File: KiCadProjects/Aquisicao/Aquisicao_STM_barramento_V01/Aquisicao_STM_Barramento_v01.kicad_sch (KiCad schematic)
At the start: 13 parts, among them J1 alimentacao analogica, J2 sinais analogicos, J3 comunicacao / sinais digitais, J4 Conn_01x02, U1 BluePill_STM32F103C, U2 LM2596S-5, U3 LM1117T-3.3

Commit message: modificar
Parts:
- added J5: Conn_01x02, symbol Connector_Generic:Conn_01x02
- added U4, U5, U6: BluePill_STM32F103C, BluePill_breakouts:BluePill_STM32F103C, symbol bluepill_breakouts:BluePill_STM32F103C
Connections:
- net 3.3V_step: now also U4.40 (VCC3V3), U5.40 (VCC3V3), U6.40 (VCC3V3)
- net Ampl1: now also U1.6 (PA1), U4.6 (PA1), U5.6 (PA1), U6.6 (PA1); no longer U1.13 (PB0)
- net Ampl2: now also U1.9 (PA4), U4.9 (PA4), U5.9 (PA4), U6.9 (PA4); no longer U1.14 (PB1)
- net Earth: now also U4.20 (GND), U5.20 (GND), U6.20 (GND)
- net SCL1: now also U4.36 (PB8), U5.36 (PB8), U6.36 (PB8)
- net SDA1: now also U4.37 (PB9), U5.37 (PB9), U6.37 (PB9)
- net SINCD: now also U1.3 (PC14), U4.3 (PC14), U5.3 (PC14), U6.3 (PC14)
- net SINC_A: now also U1.10 (PA5_SCK1), U4.10 (PA5_SCK1), U5.10 (PA5_SCK1), U6.10 (PA5_SCK1)
- net SINC_B: now also U1.11 (PA6_MISO1), U4.11 (PA6_MISO1), U5.11 (PA6_MISO1), U6.11 (PA6_MISO1)
- net SINC_C: now also U1.12 (PA7_MOSI1), U4.12 (PA7_MOSI1), U5.12 (PA7_MOSI1), U6.12 (PA7_MOSI1)
- net sign_E1: now also U4.5 (PA0)
- new net sign_E2: J5.1 (Pin_1), U5.5 (PA0)
- new net sign_E3: J5.2 (Pin_2), U6.5 (PA0)
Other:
- moved on the sheet: J4, U1

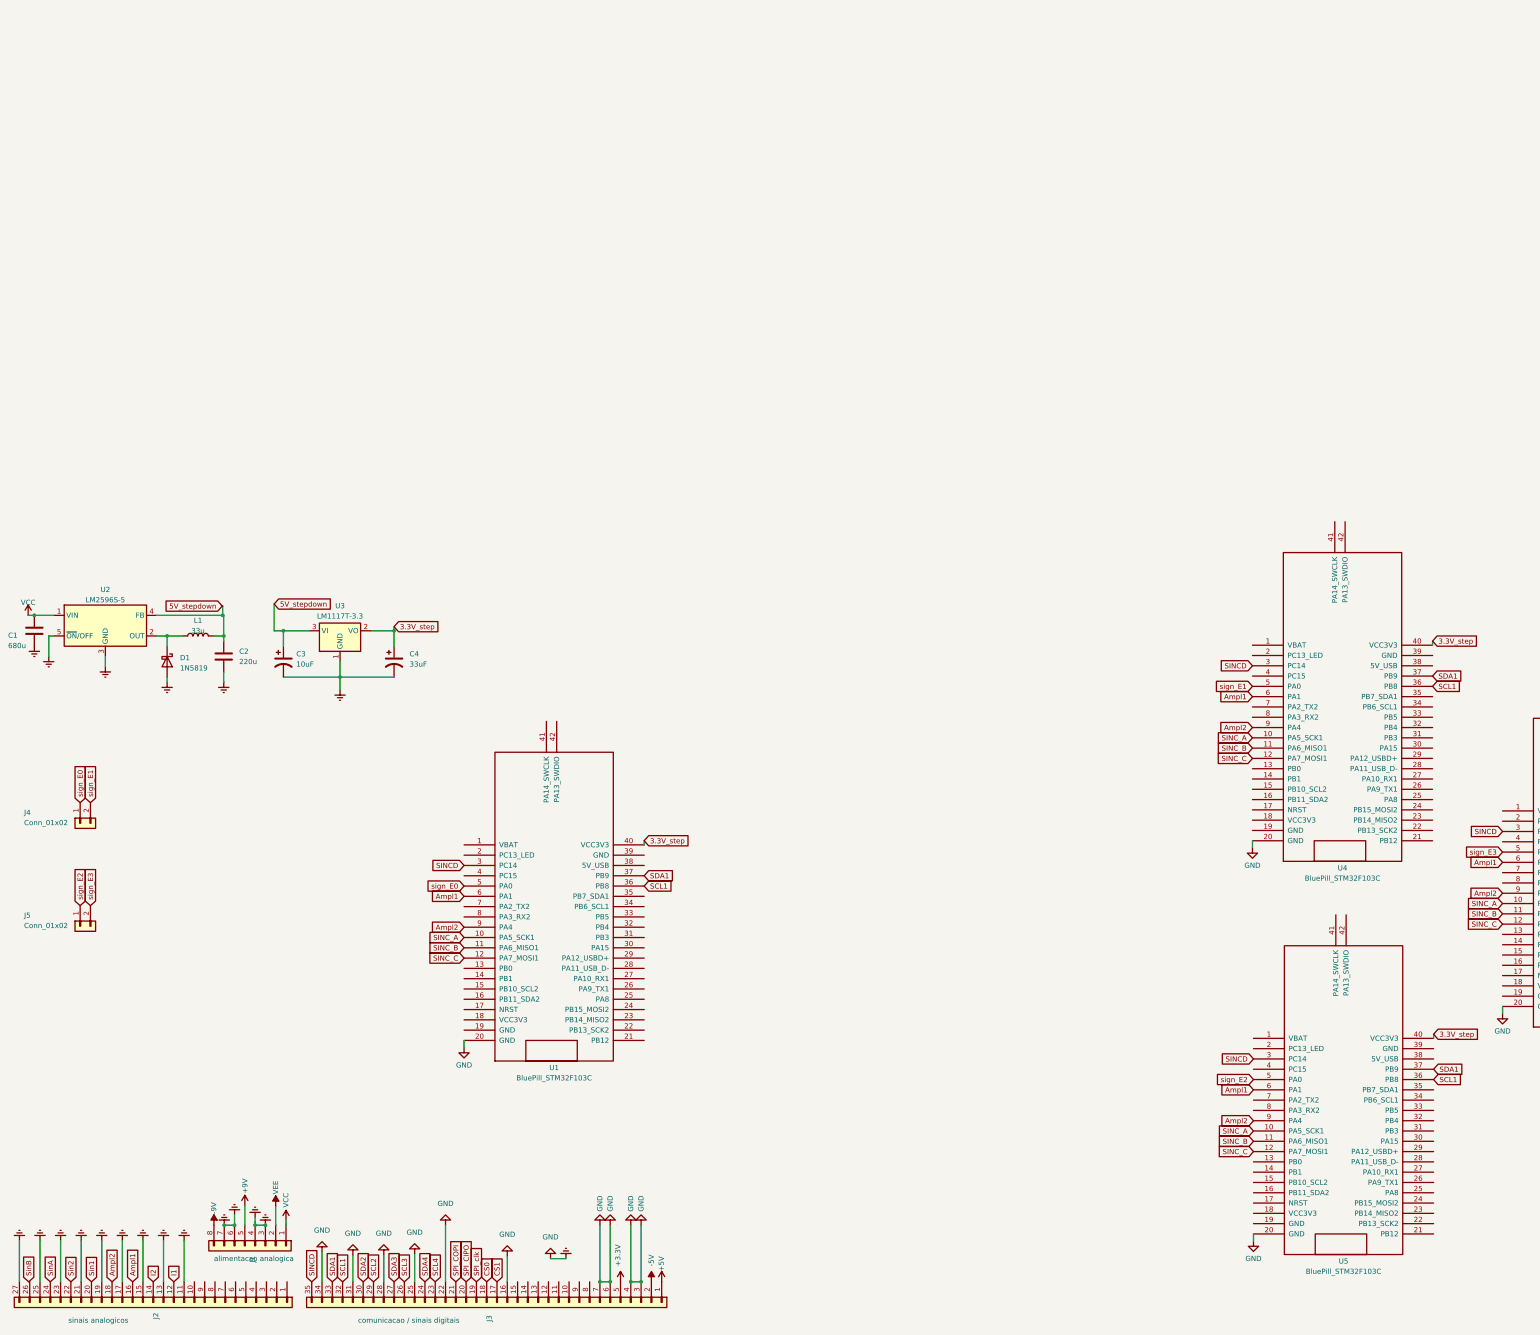
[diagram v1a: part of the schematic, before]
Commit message: tmp
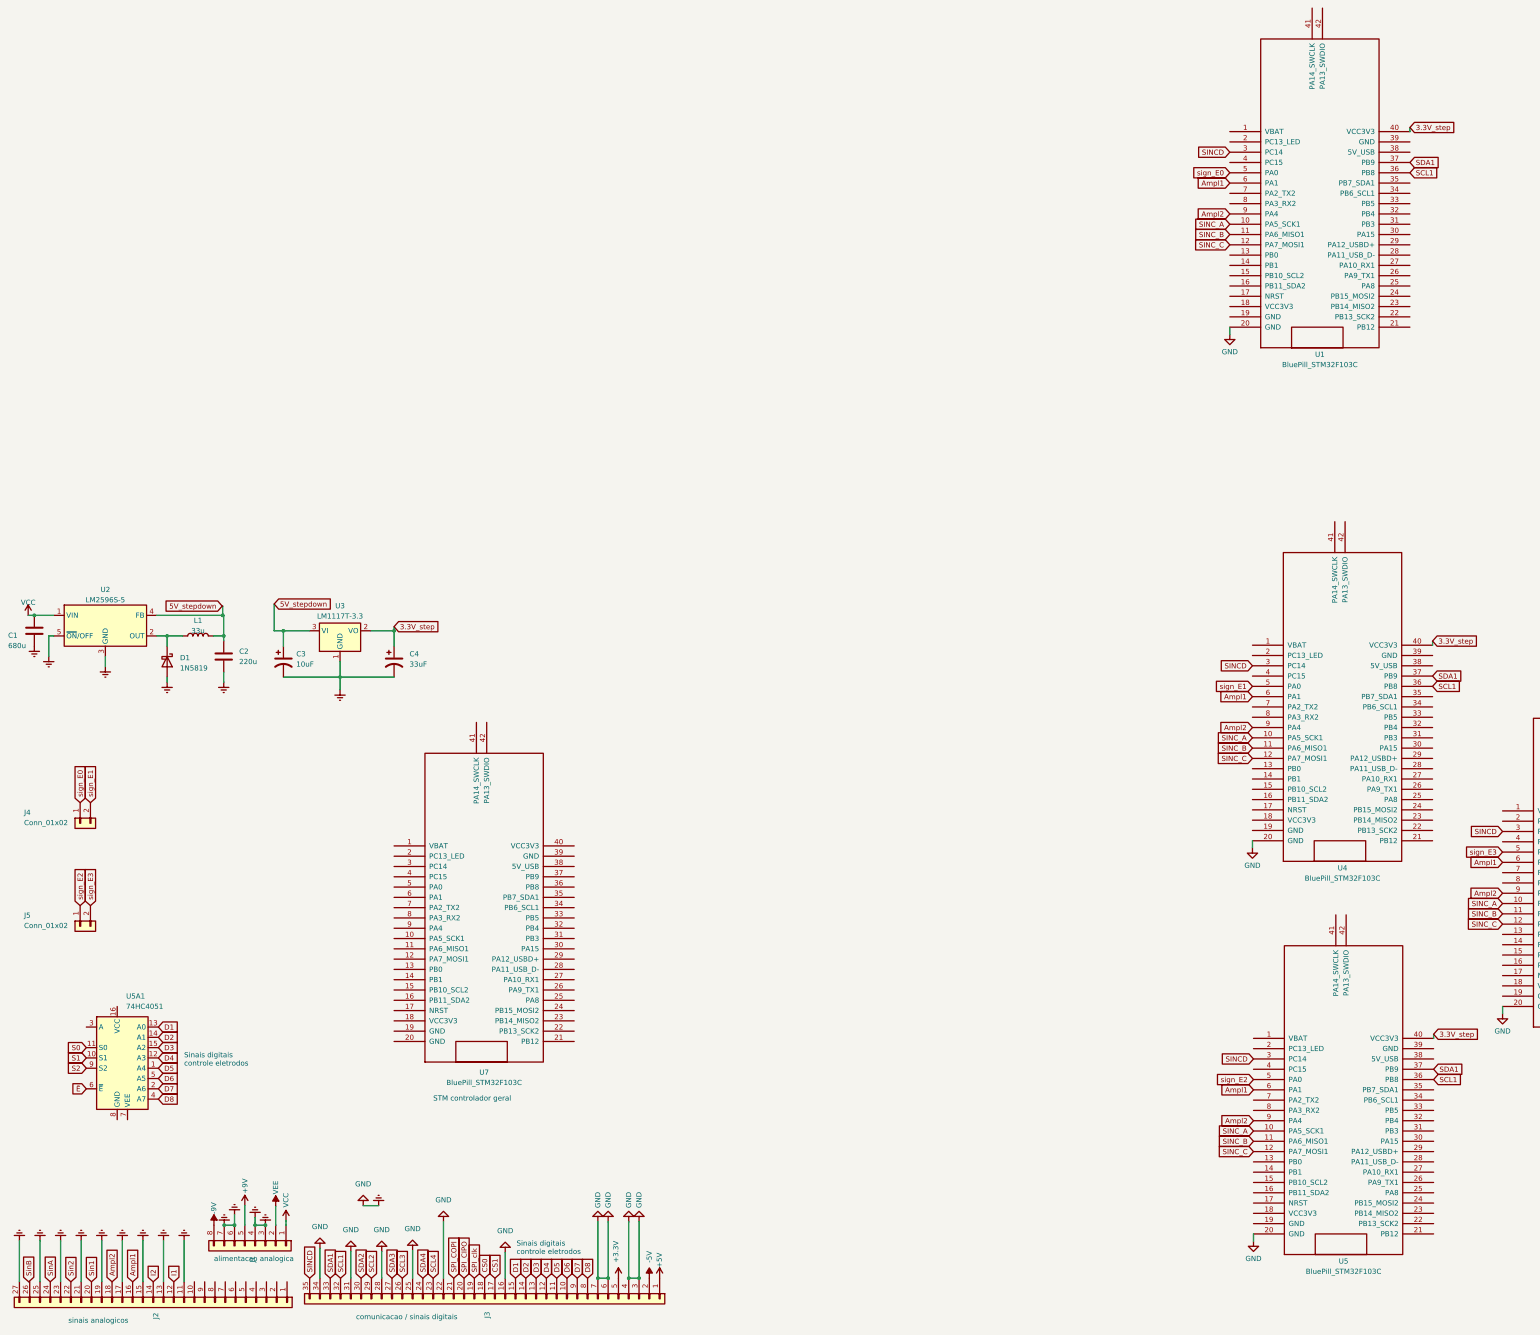
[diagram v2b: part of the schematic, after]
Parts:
- added U5A1: 74HC4051, 74HC4051N:N16, symbol 74xx:74HC4051
- added U7: BluePill_STM32F103C, BluePill_breakouts:BluePill_STM32F103C, symbol bluepill_breakouts:BluePill_STM32F103C
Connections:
- net D6: now reaches J3.10 (Pin_10)
- net D6: now also U5A1.5 (A5)
- net D5: now reaches J3.11 (Pin_11)
- net D5: now also U5A1.1 (A4)
- net D4: now reaches J3.12 (Pin_12)
- net D4: now also U5A1.12 (A3)
- net D3: now reaches J3.13 (Pin_13)
- net D3: now also U5A1.15 (A2)
- net D2: now reaches J3.14 (Pin_14)
- net D2: now also U5A1.14 (A1)
- net D1: now reaches J3.15 (Pin_15)
- net D1: now also U5A1.13 (A0)
- net D8: now reaches J3.8 (Pin_8)
- net D8: now also U5A1.4 (A7)
- net D7: now reaches J3.9 (Pin_9)
- net D7: now also U5A1.2 (A6)
- new net S0: U5A1.11 (S0)
- new net S1: U5A1.10 (S1)
- new net S2: U5A1.9 (S2)
- new net Ẽ: U5A1.6 (~{E})
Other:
- note added: "STM controlador geral"
- note added: "Sinais digitais controle eletrodos"
- moved on the sheet: J3, U1

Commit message: tmp
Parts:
- removed U5A1: 74HC4051, 74HC4051N:N16, symbol 74xx:74HC4051
- removed U7: BluePill_STM32F103C, BluePill_breakouts:BluePill_STM32F103C, symbol bluepill_breakouts:BluePill_STM32F103C
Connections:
- net D1 is gone; now on net SINC_A: J3.15 (Pin_15)
- net D2 is gone; now on net SINC_B: J3.14 (Pin_14)
- net D3 is gone; now on net SINC_C: J3.13 (Pin_13)
- net SCL1: now also U1.34 (PB6_SCL1), U4.34 (PB6_SCL1), U5.34 (PB6_SCL1), U6.34 (PB6_SCL1); no longer U1.36 (PB8), U4.36 (PB8), U5.36 (PB8), U6.36 (PB8)
- net SDA1: now also U1.35 (PB7_SDA1), U4.35 (PB7_SDA1), U5.35 (PB7_SDA1), U6.35 (PB7_SDA1); no longer U1.37 (PB9), U4.37 (PB9), U5.37 (PB9), U6.37 (PB9)
- net D4: no longer names the net of J3.12 (Pin_12)
- net D5: no longer names the net of J3.11 (Pin_11)
- net D6: no longer names the net of J3.10 (Pin_10)
- net D7: no longer names the net of J3.9 (Pin_9)
- net D8: no longer names the net of J3.8 (Pin_8)
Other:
- note removed: "STM controlador geral"
- note removed: "Sinais digitais controle eletrodos"
- moved on the sheet: C1, C2, C3, C4, D1, J4, J5, L1, U1, U2, U3, U4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
